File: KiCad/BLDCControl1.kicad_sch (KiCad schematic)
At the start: 37 parts, among them J2 Conn_Power, J3 Conn BLDC, Q1 IRLZ44N, Q2 IRLZ44N, Q3 IRLZ44N, Q4 IRLZ44N, Q5 IRLZ44N, Q6 IRLZ44N, U1 IR2101, U2 IR2101, U3 IR2101, U4 YAAJ_BlackPill_v2, U5 L7805, U6 LM339

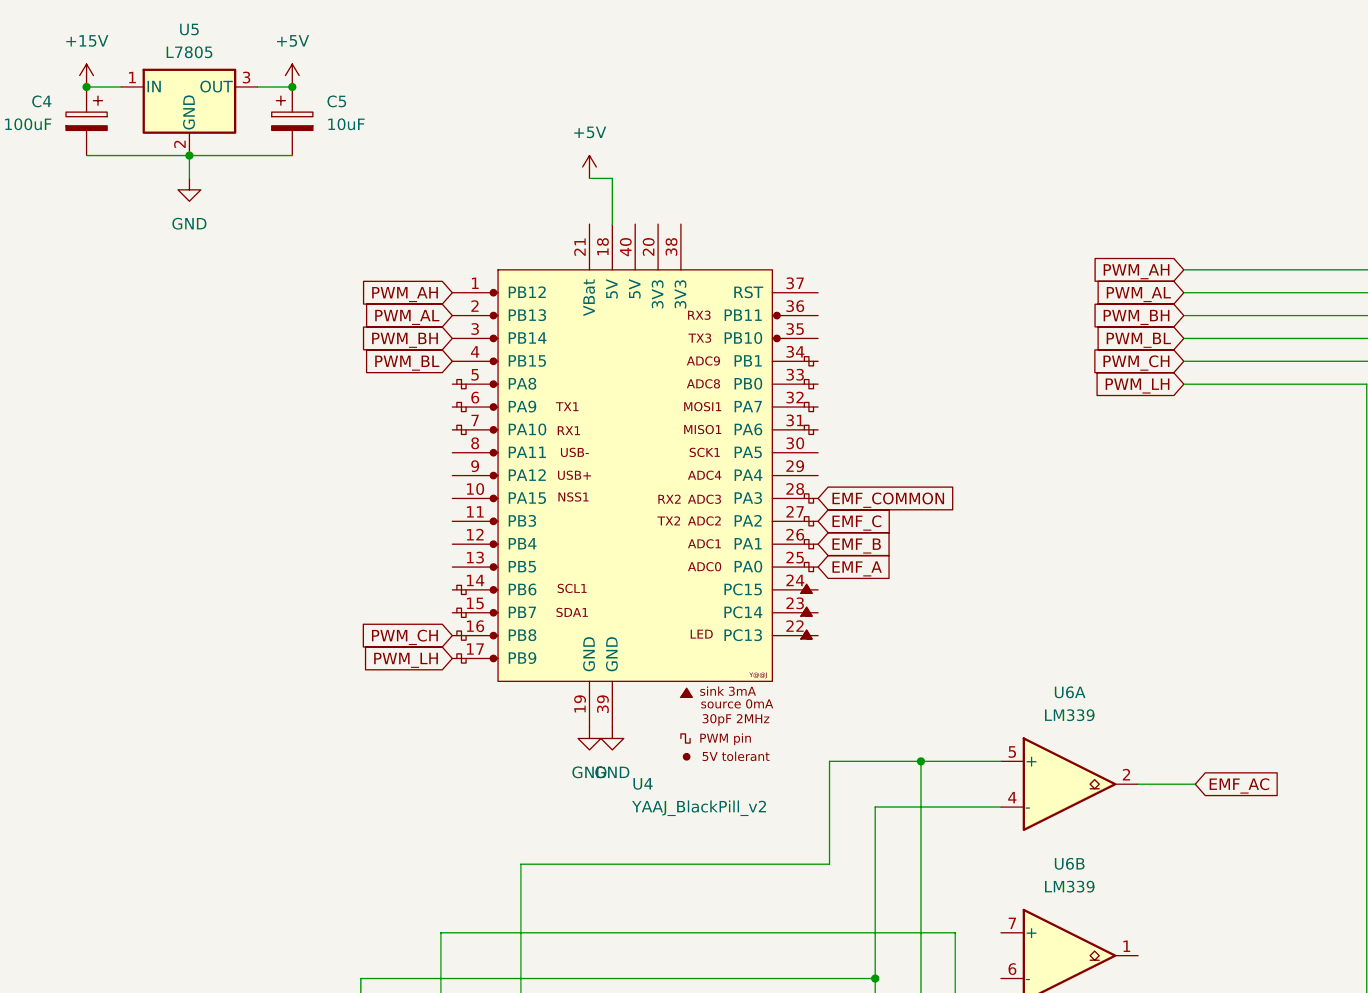
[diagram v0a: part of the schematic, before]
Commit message: i2c
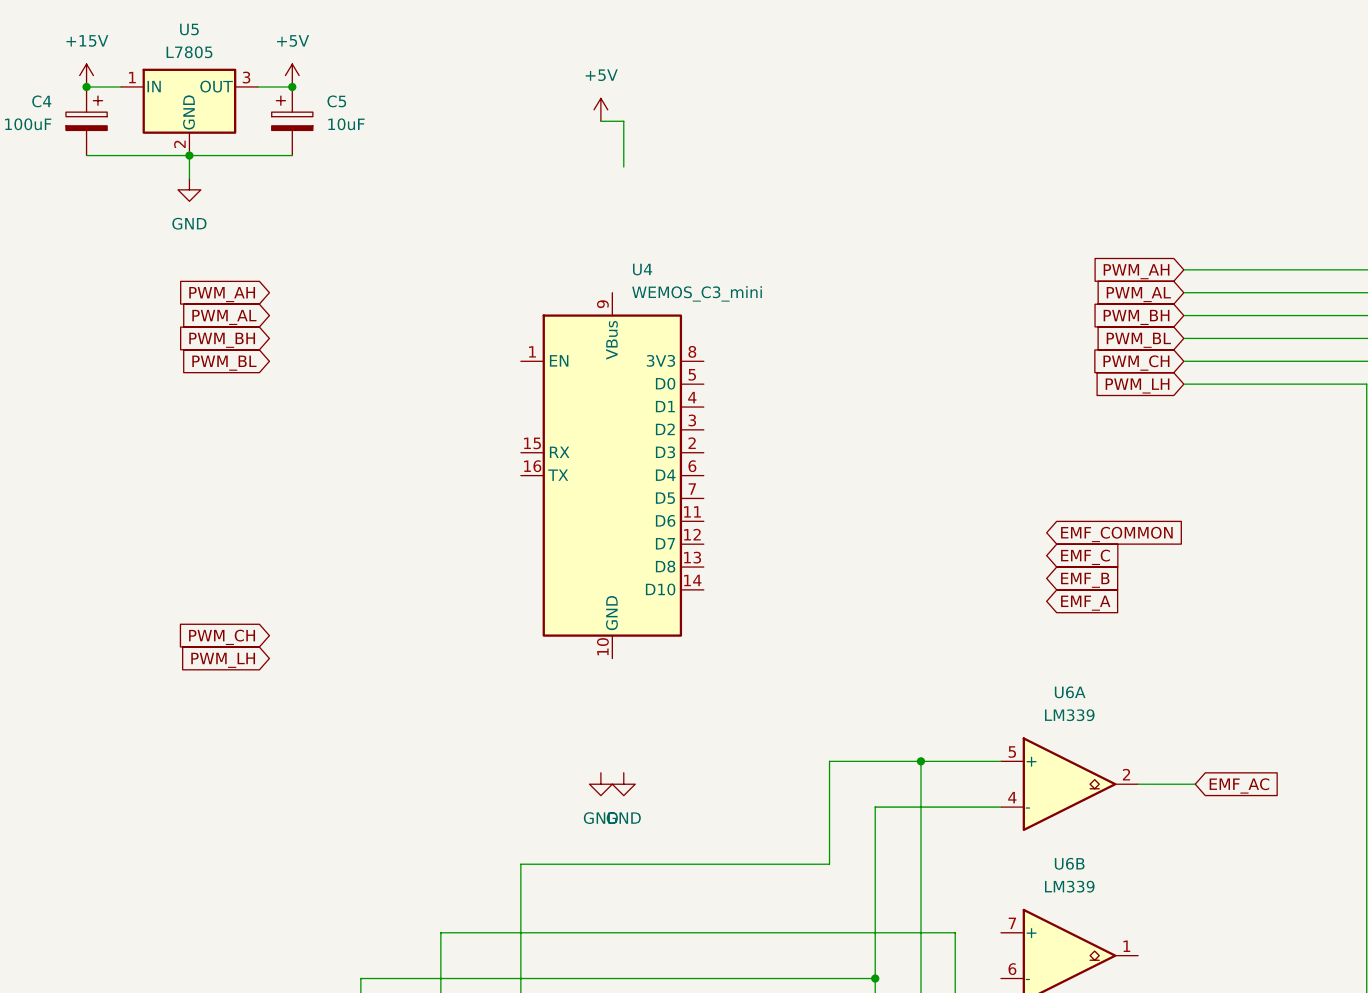
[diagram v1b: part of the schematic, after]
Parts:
- removed U4: YAAJ_BlackPill_v2, Package_DIP:DIP-40_W15.24mm, symbol YAAJ_BluePill:YAAJ_BlackPill_v2
- added U4: WEMOS_C3_mini, RF_Module:WEMOS_C3_mini, symbol RF_Module:WEMOS_C3_mini
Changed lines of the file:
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@@
 	(wire
 		(pts
-			(xy 80.01 43.18) (xy 82.55 43.18)
+			(xy 81.28 36.83) (xy 83.82 36.83)
 		)
 		(stroke
@@
 	(wire
 		(pts
-			(xy 82.55 43.18) (xy 82.55 48.26)
+			(xy 83.82 36.83) (xy 83.82 41.91)
 		)
 		(stroke
@@
 	(global_label "EMF_COMMON"
 		(shape input)
-		(at 105.41 78.74 0)
+		(at 130.81 82.55 0)
 		(fields_autoplaced yes)
 		(effects
@@
 		)
 		(property "Intersheetrefs" "${INTERSHEET_REFS}"
-			(at 114.3218 78.74 0)
+			(at 139.7218 82.55 0)
 			(effects
 				(font
@@
 	(global_label "PWM_AH"
 		(shape input)
-		(at 64.77 55.88 180)
+		(at 44.45 55.88 180)
 		(fields_autoplaced yes)
 		(effects
@@
 		)
 		(property "Intersheetrefs" "${INTERSHEET_REFS}"
-			(at 54.2253 55.88 0)
+			(at 33.9053 55.88 0)
 			(effects
 				(font
@@
 	(global_label "EMF_C"
 		(shape input)
-		(at 105.41 81.28 0)
+		(at 130.81 85.09 0)
 		(fields_autoplaced yes)
 		(effects
@@
 		)
 		(property "Intersheetrefs" "${INTERSHEET_REFS}"
-			(at 114.1404 81.28 0)
+			(at 139.5404 85.09 0)
 			(effects
 				(font
@@
 	(global_label "PWM_CH"
 		(shape input)
-		(at 64.77 93.98 180)
+		(at 44.45 93.98 180)
 		(fields_autoplaced yes)
 		(effects
@@
 		)
 		(property "Intersheetrefs" "${INTERSHEET_REFS}"
-			(at 54.2253 93.98 0)
+			(at 33.9053 93.98 0)
 			(effects
 				(font
@@
 	(global_label "EMF_B"
 		(shape input)
-		(at 105.41 83.82 0)
+		(at 130.81 87.63 0)
 		(fields_autoplaced yes)
 		(effects
@@
 		)
 		(property "Intersheetrefs" "${INTERSHEET_REFS}"
-			(at 114.1404 83.82 0)
+			(at 139.5404 87.63 0)
 			(effects
 				(font
@@
 	(global_label "PWM_LH"
 		(shape input)
-		(at 64.77 96.52 180)
+		(at 44.45 96.52 180)
 		(fields_autoplaced yes)
 		(effects
@@
 		)
 		(property "Intersheetrefs" "${INTERSHEET_REFS}"
-			(at 54.2253 96.52 0)
+			(at 33.9053 96.52 0)
 			(effects
 				(font
@@
 	(global_label "PWM_BH"
 		(shape input)
-		(at 64.77 60.96 180)
+		(at 44.45 60.96 180)
 		(fields_autoplaced yes)
 		(effects
@@
 		)
 		(property "Intersheetrefs" "${INTERSHEET_REFS}"
-			(at 54.2253 60.96 0)
+			(at 33.9053 60.96 0)
 			(effects
 				(font
@@
 	(global_label "EMF_A"
 		(shape input)
-		(at 105.41 86.36 0)
+		(at 130.81 90.17 0)
 		(fields_autoplaced yes)
 		(effects
@@
 		)
 		(property "Intersheetrefs" "${INTERSHEET_REFS}"
-			(at 114.1404 86.36 0)
+			(at 139.5404 90.17 0)
 			(effects
 				(font
@@
 	(global_label "PWM_AL"
 		(shape input)
-		(at 64.77 58.42 180)
+		(at 44.45 58.42 180)
 		(fields_autoplaced yes)
 		(effects
@@
 		)
 		(property "Intersheetrefs" "${INTERSHEET_REFS}"
-			(at 54.2253 58.42 0)
+			(at 33.9053 58.42 0)
 			(effects
 				(font
@@
 	(global_label "PWM_BL"
 		(shape input)
-		(at 64.77 63.5 180)
+		(at 44.45 63.5 180)
 		(fields_autoplaced yes)
 		(effects
@@
 		)
 		(property "Intersheetrefs" "${INTERSHEET_REFS}"
-			(at 54.2253 63.5 0)
+			(at 33.9053 63.5 0)
 			(effects
 				(font
@@
 	(symbol
 		(lib_id "power:GND")
-		(at 80.01 104.14 0)
+		(at 81.28 109.22 0)
 		(unit 1)
 		(exclude_from_sim no)
@@
 		(fields_autoplaced yes)
 		(property "Reference" "#PWR014"
-			(at 80.01 110.49 0)
+			(at 81.28 115.57 0)
 			(effects
 				(font
@@
 		)
 		(property "Value" "GND"
-			(at 80.01 109.22 0)
+			(at 81.28 114.3 0)
 			(effects
 				(font
@@
 		)
 		(property "Footprint" ""
-			(at 80.01 104.14 0)
+			(at 81.28 109.22 0)
 			(effects
 				(font
@@
 		)
 		(property "Datasheet" ""
-			(at 80.01 104.14 0)
+			(at 81.28 109.22 0)
 			(effects
 				(font
@@
 		)
 		(property "Description" "Power symbol creates a global label with name \"GND\" , ground"
-			(at 80.01 104.14 0)
+			(at 81.28 109.22 0)
 			(effects
 				(font
@@
 	)
 	(symbol
-		(lib_id "YAAJ_BluePill:YAAJ_BlackPill_v2")
-		(at 85.09 76.2 0)
+		(lib_id "RF_Module:WEMOS_C3_mini")
+		(at 82.55 76.2 0)
 		(unit 1)
 		(exclude_from_sim no)
@@
 		(fields_autoplaced yes)
 		(property "Reference" "U4"
-			(at 84.7441 110.49 0)
+			(at 84.6933 53.34 0)
 			(effects
 				(font
@@
 			)
 		)
-		(property "Value" "YAAJ_BlackPill_v2"
-			(at 84.7441 113.03 0)
+		(property "Value" "WEMOS_C3_mini"
+			(at 84.6933 55.88 0)
 			(effects
 				(font
@@
 			)
 		)
-		(property "Footprint" "Package_DIP:DIP-40_W15.24mm"
-			(at 83.185 52.07 90)
+		(property "Footprint" "RF_Module:WEMOS_C3_mini"
+			(at 82.55 105.41 0)
 			(effects
 				(font
@@
 			)
 		)
-		(property "Datasheet" ""
-			(at 83.185 52.07 90)
+		(property "Datasheet" "https://www.wemos.cc/en/latest/c3/c3_mini.html"
+			(at 82.55 102.616 0)
 			(effects
 				(font
@@
 			)
 		)
-		(property "Description" "STM32 Blue Pill ; KLC compliant"
-			(at 85.09 76.2 0)
+		(property "Description" "32-bit microcontroller module with WiFi"
+			(at 83.312 99.314 0)
 			(effects
 				(font
@@
 			)
 		)
-		(pin "36"
-		)
-		(pin "20"
-		)
-		(pin "28"
-		)
-		(pin "11"
-		)
-		(pin "4"
-		)
-		(pin "22"
-		)
-		(pin "25"
+		(pin "14"
 		)
-		(pin "26"
+		(pin "7"
 		)
-		(pin "9"
+		(pin "16"
 		)
-		(pin "31"
+		(pin "2"
 		)
-		(pin "34"
+		(pin "11"
 		)
 		(pin "12"
 		)
-		(pin "14"
-		)
 		(pin "15"
 		)
-		(pin "32"
-		)
-		(pin "5"
-		)
-		(pin "13"
-		)
-		(pin "3"
-		)
-		(pin "21"
-		)
-		(pin "27"
-		)
-		(pin "8"
-		)
-		(pin "10"
-		)
-		(pin "16"
-		)
-		(pin "7"
+		(pin "9"
 		)
 		(pin "1"
 		)
-		(pin "39"
-		)
-		(pin "17"
-		)
-		(pin "18"
-		)
-		(pin "35"
-		)
-		(pin "23"
-		)
-		(pin "38"
-		)
-		(pin "40"
-		)
-		(pin "24"
-		)
-		(pin "19"
-		)
-		(pin "30"
+		(pin "4"
 		)
-		(pin "2"
+		(pin "8"
 		)
-		(pin "29"
+		(pin "5"
 		)
-		(pin "33"
+		(pin "10"
 		)
-		(pin "37"
+		(pin "3"
 		)
 		(pin "6"
 		)
+		(pin "13"
+		)
 		(instances
 			(project ""
@@
 	(symbol
 		(lib_id "power:GND")
-		(at 82.55 104.14 0)
+		(at 83.82 109.22 0)
 		(unit 1)
 		(exclude_from_sim no)
@@
 		(fields_autoplaced yes)
 		(property "Reference" "#PWR015"
-			(at 82.55 110.49 0)
+			(at 83.82 115.57 0)
 			(effects
 				(font
@@
 		)
 		(property "Value" "GND"
-			(at 82.55 109.22 0)
+			(at 83.82 114.3 0)
 			(effects
 				(font
@@
 		)
 		(property "Footprint" ""
-			(at 82.55 104.14 0)
+			(at 83.82 109.22 0)
 			(effects
 				(font
@@
 		)
 		(property "Datasheet" ""
-			(at 82.55 104.14 0)
+			(at 83.82 109.22 0)
 			(effects
 				(font
@@
 		)
 		(property "Description" "Power symbol creates a global label with name \"GND\" , ground"
-			(at 82.55 104.14 0)
+			(at 83.82 109.22 0)
 			(effects
 				(font
@@
 	(symbol
 		(lib_id "power:+5V")
-		(at 80.01 43.18 0)
+		(at 81.28 36.83 0)
 		(unit 1)
 		(exclude_from_sim no)
@@
 		(fields_autoplaced yes)
 		(property "Reference" "#PWR016"
-			(at 80.01 46.99 0)
+			(at 81.28 40.64 0)
 			(effects
 				(font
@@
 		)
 		(property "Value" "+5V"
-			(at 80.01 38.1 0)
+			(at 81.28 31.75 0)
 			(effects
 				(font
@@
 		)
 		(property "Footprint" ""
-			(at 80.01 43.18 0)
+			(at 81.28 36.83 0)
 			(effects
 				(font
@@
 		)
 		(property "Datasheet" ""
-			(at 80.01 43.18 0)
+			(at 81.28 36.83 0)
 			(effects
 				(font
@@
 		)
 		(property "Description" "Power symbol creates a global label with name \"+5V\""
-			(at 80.01 43.18 0)
+			(at 81.28 36.83 0)
 			(effects
 				(font
